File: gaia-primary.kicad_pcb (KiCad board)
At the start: 4 copper layers, 50 x 50 mm, 66 parts, among them IC2 ADXL375BCCZ, J1 Debug Connectors, J2 Conn_02x10_Odd_Even, J3 Conn_02x10_Odd_Even, Q1 BSS138, Q2 BSS138, U10 AP2112K-1.8, U11 AP2112K-3.3, U12 ICM-20948, U13 ICM-20948, U4 STM32F103C8Tx, U5 MAX31865xTP, U6 BME680/BME690, U7 MAX31865xTP, U9 BME680/BME690, Y1 Crystal

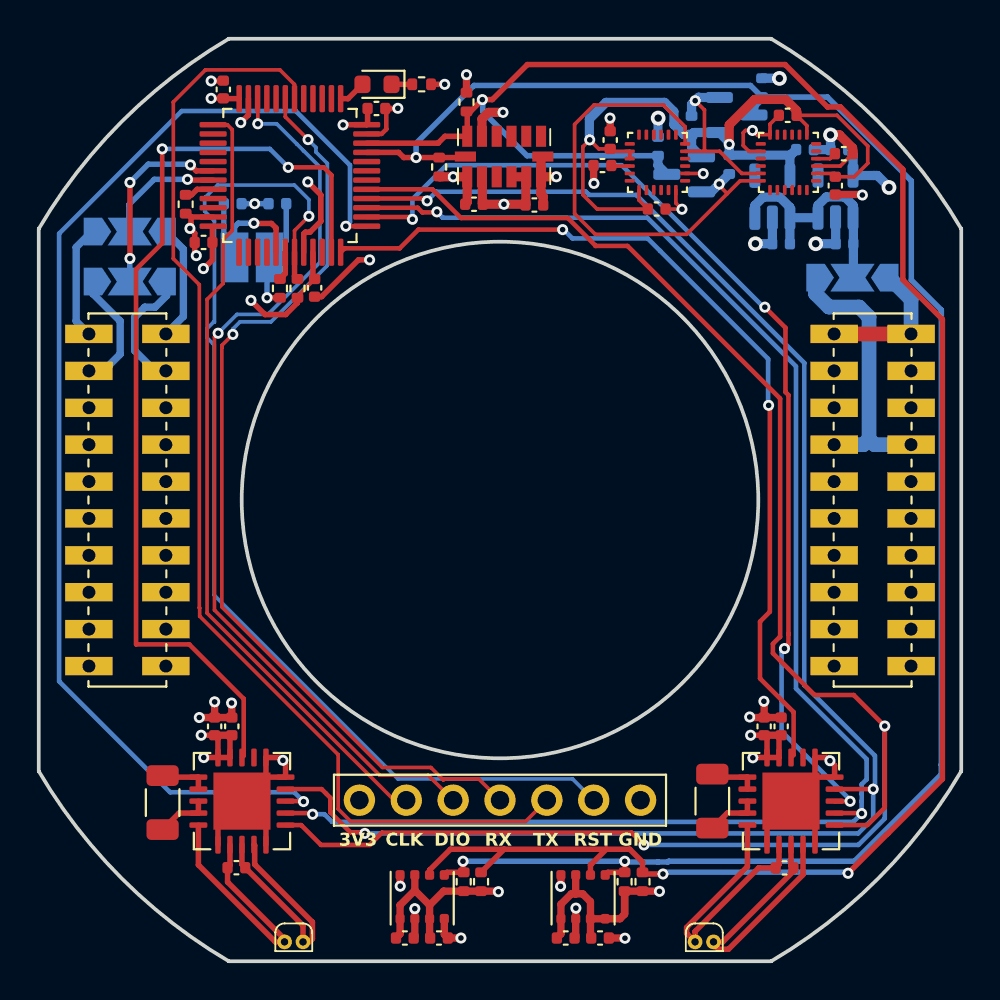
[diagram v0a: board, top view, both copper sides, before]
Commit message: Update gaia-primary.kicad_pcb
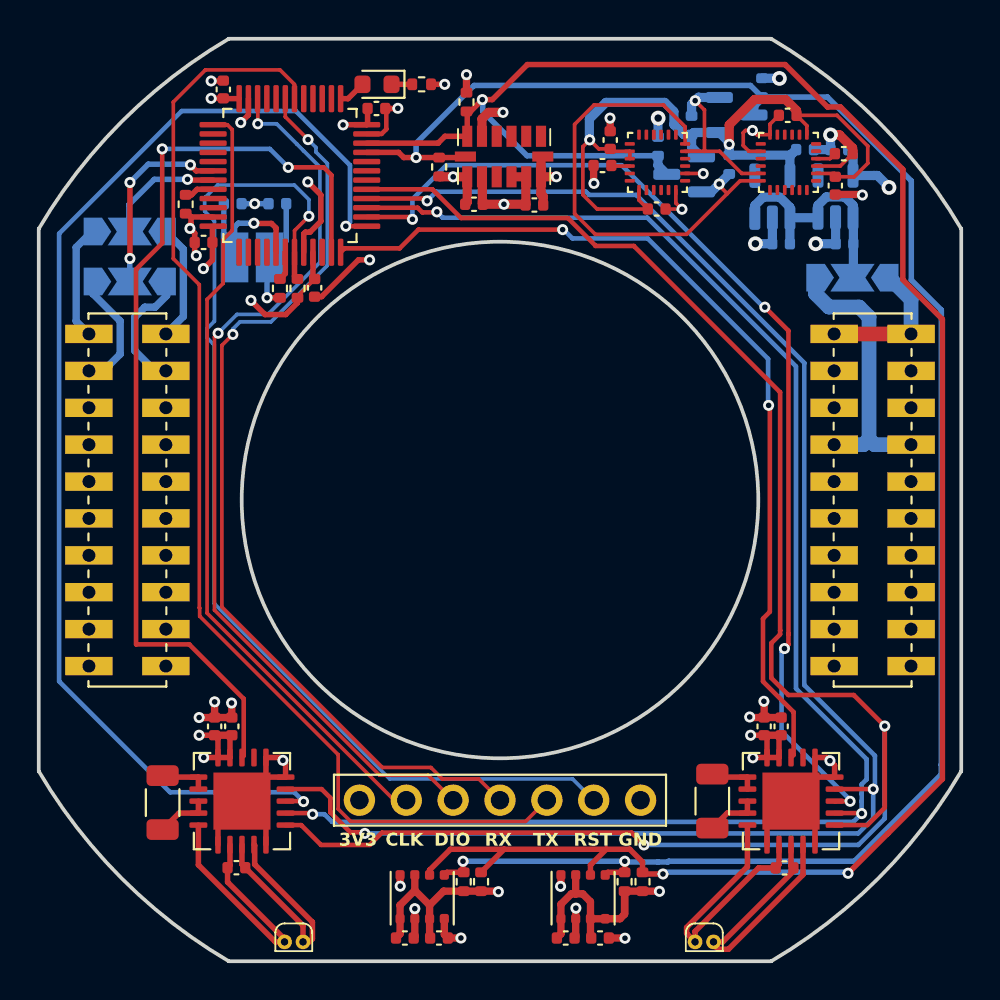
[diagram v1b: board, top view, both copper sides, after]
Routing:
- net /SPI1_MOSI: track 95.4 -> 96.5 mm
